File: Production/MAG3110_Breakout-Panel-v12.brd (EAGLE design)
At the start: 123.4 x 123.4 mm, 836 parts, among them U1 MAG31101:1, U10 MAG31101:1, U11 MAG31101:1, U12 MAG31101:1, U13 MAG31101:1, U14 MAG31101:1, U15 MAG31101:1, U16 MAG31101:1, U17 MAG31101:1, U18 MAG31101:1, U19 MAG31101:1, U2 MAG31101:1, U20 MAG31101:1, U21 MAG31101:1, U22 MAG31101:1, U23 MAG31101:1, U24 MAG31101:1, U25 MAG31101:1, U26 MAG31101:1, U27 MAG31101:1, U28 MAG31101:1, U29 MAG31101:1, U3 MAG31101:1, U30 MAG31101:1, U31 MAG31101:1, U32 MAG31101:1, U33 MAG31101:1, U34 MAG31101:1, U35 MAG31101:1, U36 MAG31101:1, U37 MAG31101:1, U38 MAG31101:1, U39 MAG31101:1, U4 MAG31101:1, U40 MAG31101:1, U41 MAG31101:1, U42 MAG31101:1, U43 MAG31101:1, U44 MAG31101:1, U45 MAG31101:1, U46 MAG31101:1, U47 MAG31101:1, U48 MAG31101:1, U49 MAG31101:1, U5 MAG31101:1, U6 MAG31101:1, U7 MAG31101:1, U8 MAG31101:1, U9 MAG31101:1

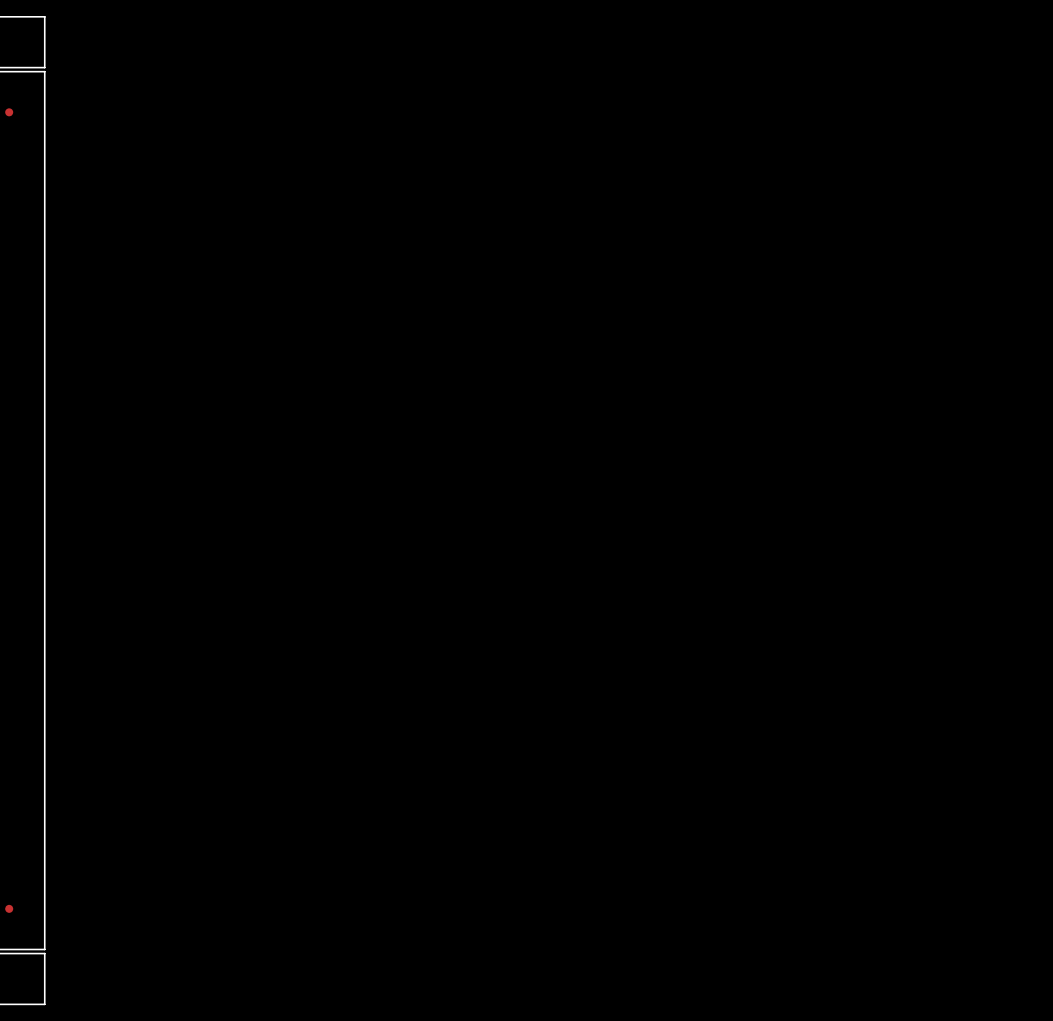
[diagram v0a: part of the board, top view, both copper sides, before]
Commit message: made larger panel
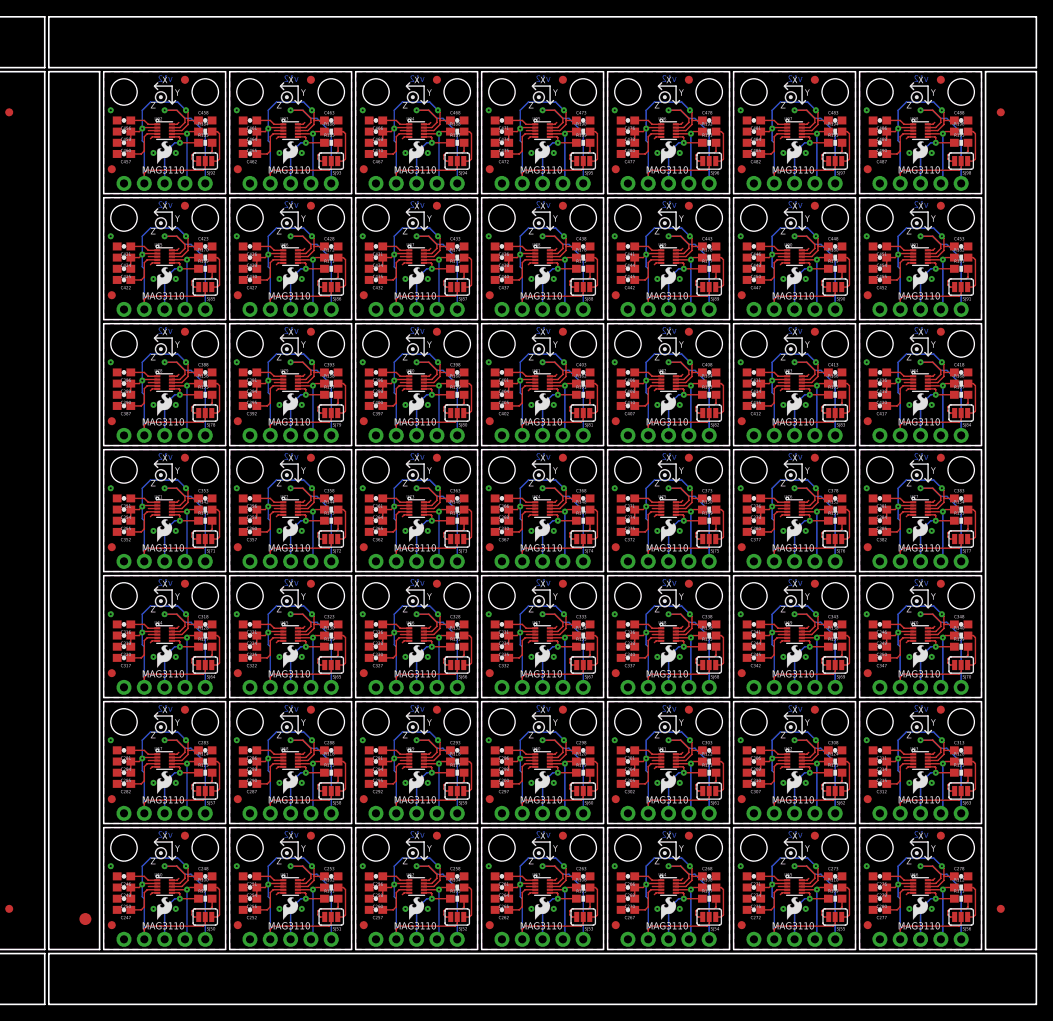
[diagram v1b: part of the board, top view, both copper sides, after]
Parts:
- added C246, C247, C248, C250, C251, C252, C253, C255, C256, C257, C258, C260, C261, C262, C263, C265, C266, C267, C268, C270, C271, C272, C273, C275, C276, C277, C278, C280, C281, C282, C283, C285, C286, C287, C288, C290, C291, C292, C293, C295, C296, C297, C298, C300, C301, C302, C303, C305, C306, C307, C308, C310, C311, C312, C313, C315, C316, C317, C318, C320, C321, C322, C323, C325, C326, C327, C328, C330, C331, C332, C333, C335, C336, C337, C338, C340, C341, C342, C343, C345, C346, C347, C348, C350, C351, C352, C353, C355, C356, C357, C358, C360, C361, C362, C363, C365, C366, C367, C368, C370, C371, C372, C373, C375, C376, C377, C378, C380, C381, C382, C383, C385, C386, C387, C388, C390, C391, C392, C393, C395, C396, C397, C398, C400, C401, C402, C403, C405, C406, C407, C408, C410, C411, C412, C413, C415, C416, C417, C418, C420, C421, C422, C423, C425, C426, C427, C428, C430, C431, C432, C433, C435, C436, C437, C438, C440, C441, C442, C443, C445, C446, C447, C448, C450, C451, C452, C453, C455, C456, C457, C458, C460, C461, C462, C463, C465, C466, C467, C468, C470, C471, C472, C473, C475, C476, C477, C478, C480, C481, C482, C483, C485, C486, C487, C488, C490: 0.1uF, SparkFun:0603-CAP
- added C249, C254, C259, C264, C269, C274, C279, C284, C289, C294, C299, C304, C309, C314, C319, C324, C329, C334, C339, C344, C349, C354, C359, C364, C369, C374, C379, C384, C389, C394, C399, C404, C409, C414, C419, C424, C429, C434, C439, C444, C449, C454, C459, C464, C469, C474, C479, C484, C489: 1uF, SparkFun:0603-CAP
- added E$2, E$3: (no value), SparkFun-Aesthetics:FIDUCIAL-1X2
- added E$5: (no value), SparkFun-Retired:FIDUCIAL-1.5X3
- added FID100, FID101, FID102, FID103, FID104, FID105, FID106, FID107, FID108, FID109, FID110, FID111, FID112, FID113, FID114, FID115, FID116, FID117, FID118, FID119, FID120, FID121, FID122, FID123, FID124, FID125, FID126, FID127, FID128, FID129, FID130, FID131, FID132, FID133, FID134, FID135, FID136, FID137, FID138, FID139, FID140, FID141, FID142, FID143, FID144, FID145, FID146, FID147, FID148, FID149, FID150, FID151, FID152, FID153, FID154, FID155, FID156, FID157, FID158, FID159, FID160, FID161, FID162, FID163, FID164, FID165, FID166, FID167, FID168, FID169, FID170, FID171, FID172, FID173, FID174, FID175, FID176, FID177, FID178, FID179, FID180, FID181, FID182, FID183, FID184, FID185, FID186, FID187, FID188, FID189, FID190, FID191, FID192, FID193, FID194, FID195, FID196, FID99: FIDUCIAL1X2, SparkFun-Aesthetics:FIDUCIAL-1X2
- added JP246, JP251, JP256, JP261, JP266, JP271, JP276, JP281, JP286, JP291, JP296, JP301, JP306, JP311, JP316, JP321, JP326, JP331, JP336, JP341, JP346, JP351, JP356, JP361, JP366, JP371, JP376, JP381, JP386, JP391, JP396, JP401, JP406, JP411, JP416, JP421, JP426, JP431, JP436, JP441, JP446, JP451, JP456, JP461, JP466, JP471, JP476, JP481, JP486: breakout, SparkFun:1X05
- added JP247, JP248, JP252, JP253, JP257, JP258, JP262, JP263, JP267, JP268, JP272, JP273, JP277, JP278, JP282, JP283, JP287, JP288, JP292, JP293, JP297, JP298, JP302, JP303, JP307, JP308, JP312, JP313, JP317, JP318, JP322, JP323, JP327, JP328, JP332, JP333, JP337, JP338, JP342, JP343, JP347, JP348, JP352, JP353, JP357, JP358, JP362, JP363, JP367, JP368, JP372, JP373, JP377, JP378, JP382, JP383, JP387, JP388, JP392, JP393, JP397, JP398, JP402, JP403, JP407, JP408, JP412, JP413, JP417, JP418, JP422, JP423, JP427, JP428, JP432, JP433, JP437, JP438, JP442, JP443, JP447, JP448, JP452, JP453, JP457, JP458, JP462, JP463, JP467, JP468, JP472, JP473, JP477, JP478, JP482, JP483, JP487, JP488: STAND-OFF, SparkFun:STAND-OFF
- added JP249, JP250, JP254, JP255, JP259, JP260, JP264, JP265, JP269, JP270, JP274, JP275, JP279, JP280, JP284, JP285, JP289, JP290, JP294, JP295, JP299, JP300, JP304, JP305, JP309, JP310, JP314, JP315, JP319, JP320, JP324, JP325, JP329, JP330, JP334, JP335, JP339, JP340, JP344, JP345, JP349, JP350, JP354, JP355, JP359, JP360, JP364, JP365, JP369, JP370, JP374, JP375, JP379, JP380, JP384, JP385, JP389, JP390, JP394, JP395, JP399, JP400, JP404, JP405, JP409, JP410, JP414, JP415, JP419, JP420, JP424, JP425, JP429, JP430, JP434, JP435, JP439, JP440, JP444, JP445, JP449, JP450, JP454, JP455, JP459, JP460, JP464, JP465, JP469, JP470, JP474, JP475, JP479, JP480, JP484, JP485, JP489, JP490: LOGO-SFESK, SparkFun:SFE-LOGO-FLAME
- added LOGO50, LOGO51, LOGO52, LOGO53, LOGO54, LOGO55, LOGO56, LOGO57, LOGO58, LOGO59, LOGO60, LOGO61, LOGO62, LOGO63, LOGO64, LOGO65, LOGO66, LOGO67, LOGO68, LOGO69, LOGO70, LOGO71, LOGO72, LOGO73, LOGO74, LOGO75, LOGO76, LOGO77, LOGO78, LOGO79, LOGO80, LOGO81, LOGO82, LOGO83, LOGO84, LOGO85, LOGO86, LOGO87, LOGO88, LOGO89, LOGO90, LOGO91, LOGO92, LOGO93, LOGO94, LOGO95, LOGO96, LOGO97, LOGO98: OSHW-LOGOS, SparkFun-Aesthetics:OSHW-LOGO-S
- added R100, R101, R102, R103, R104, R105, R106, R107, R108, R109, R110, R111, R112, R113, R114, R115, R116, R117, R118, R119, R120, R121, R122, R123, R124, R125, R126, R127, R128, R129, R130, R131, R132, R133, R134, R135, R136, R137, R138, R139, R140, R141, R142, R143, R144, R145, R146, R147, R148, R149, R150, R151, R152, R153, R154, R155, R156, R157, R158, R159, R160, R161, R162, R163, R164, R165, R166, R167, R168, R169, R170, R171, R172, R173, R174, R175, R176, R177, R178, R179, R180, R181, R182, R183, R184, R185, R186, R187, R188, R189, R190, R191, R192, R193, R194, R195, R196, R99: 4.7k, SparkFun:0603-RES
- added SJ50, SJ51, SJ52, SJ53, SJ54, SJ55, SJ56, SJ57, SJ58, SJ59, SJ60, SJ61, SJ62, SJ63, SJ64, SJ65, SJ66, SJ67, SJ68, SJ69, SJ70, SJ71, SJ72, SJ73, SJ74, SJ75, SJ76, SJ77, SJ78, SJ79, SJ80, SJ81, SJ82, SJ83, SJ84, SJ85, SJ86, SJ87, SJ88, SJ89, SJ90, SJ91, SJ92, SJ93, SJ94, SJ95, SJ96, SJ97, SJ98: (no value), SparkFun-Passives:SJ_3_PASTE1&2&3
- added U50, U51, U52, U53, U54, U55, U56, U57, U58, U59, U60, U61, U62, U63, U64, U65, U66, U67, U68, U69, U70, U71, U72, U73, U74, U75, U76, U77, U78, U79, U80, U81, U82, U83, U84, U85, U86, U87, U88, U89, U90, U91, U92, U93, U94, U95, U96, U97, U98: MAG31101:1, SparkFun-Sensors:DFN-10-W
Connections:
- new net GND49: C246.2, C247.2, C248.2, C249.2, C250.2, JP246.1, U50.10, U50.5
- new net GND50: C251.2, C252.2, C253.2, C254.2, C255.2, JP251.1, U51.10, U51.5
- new net GND51: C256.2, C257.2, C258.2, C259.2, C260.2, JP256.1, U52.10, U52.5
- new net GND52: C261.2, C262.2, C263.2, C264.2, C265.2, JP261.1, U53.10, U53.5
- new net GND53: C266.2, C267.2, C268.2, C269.2, C270.2, JP266.1, U54.10, U54.5
- new net GND54: C271.2, C272.2, C273.2, C274.2, C275.2, JP271.1, U55.10, U55.5
- new net GND55: C276.2, C277.2, C278.2, C279.2, C280.2, JP276.1, U56.10, U56.5
- new net GND56: C281.2, C282.2, C283.2, C284.2, C285.2, JP281.1, U57.10, U57.5
- new net GND57: C286.2, C287.2, C288.2, C289.2, C290.2, JP286.1, U58.10, U58.5
- new net GND58: C291.2, C292.2, C293.2, C294.2, C295.2, JP291.1, U59.10, U59.5
- new net GND59: C296.2, C297.2, C298.2, C299.2, C300.2, JP296.1, U60.10, U60.5
- new net GND60: C301.2, C302.2, C303.2, C304.2, C305.2, JP301.1, U61.10, U61.5
- new net GND61: C306.2, C307.2, C308.2, C309.2, C310.2, JP306.1, U62.10, U62.5
- new net GND62: C311.2, C312.2, C313.2, C314.2, C315.2, JP311.1, U63.10, U63.5
- new net GND63: C316.2, C317.2, C318.2, C319.2, C320.2, JP316.1, U64.10, U64.5
- new net GND64: C321.2, C322.2, C323.2, C324.2, C325.2, JP321.1, U65.10, U65.5
- new net GND65: C326.2, C327.2, C328.2, C329.2, C330.2, JP326.1, U66.10, U66.5
- new net GND66: C331.2, C332.2, C333.2, C334.2, C335.2, JP331.1, U67.10, U67.5
- new net GND67: C336.2, C337.2, C338.2, C339.2, C340.2, JP336.1, U68.10, U68.5
- new net GND68: C341.2, C342.2, C343.2, C344.2, C345.2, JP341.1, U69.10, U69.5
- new net GND69: C346.2, C347.2, C348.2, C349.2, C350.2, JP346.1, U70.10, U70.5
- new net GND70: C351.2, C352.2, C353.2, C354.2, C355.2, JP351.1, U71.10, U71.5
- new net GND71: C356.2, C357.2, C358.2, C359.2, C360.2, JP356.1, U72.10, U72.5
- new net GND72: C361.2, C362.2, C363.2, C364.2, C365.2, JP361.1, U73.10, U73.5
- new net GND73: C366.2, C367.2, C368.2, C369.2, C370.2, JP366.1, U74.10, U74.5
- new net GND74: C371.2, C372.2, C373.2, C374.2, C375.2, JP371.1, U75.10, U75.5
- new net GND75: C376.2, C377.2, C378.2, C379.2, C380.2, JP376.1, U76.10, U76.5
- new net GND76: C381.2, C382.2, C383.2, C384.2, C385.2, JP381.1, U77.10, U77.5
- new net GND77: C386.2, C387.2, C388.2, C389.2, C390.2, JP386.1, U78.10, U78.5
- new net GND78: C391.2, C392.2, C393.2, C394.2, C395.2, JP391.1, U79.10, U79.5
- new net GND79: C396.2, C397.2, C398.2, C399.2, C400.2, JP396.1, U80.10, U80.5
- new net GND80: C401.2, C402.2, C403.2, C404.2, C405.2, JP401.1, U81.10, U81.5
- new net GND81: C406.2, C407.2, C408.2, C409.2, C410.2, JP406.1, U82.10, U82.5
- new net GND82: C411.2, C412.2, C413.2, C414.2, C415.2, JP411.1, U83.10, U83.5
- new net GND83: C416.2, C417.2, C418.2, C419.2, C420.2, JP416.1, U84.10, U84.5
- new net GND84: C421.2, C422.2, C423.2, C424.2, C425.2, JP421.1, U85.10, U85.5
- new net GND85: C426.2, C427.2, C428.2, C429.2, C430.2, JP426.1, U86.10, U86.5
- new net GND86: C431.2, C432.2, C433.2, C434.2, C435.2, JP431.1, U87.10, U87.5
- new net GND87: C436.2, C437.2, C438.2, C439.2, C440.2, JP436.1, U88.10, U88.5
- new net GND88: C441.2, C442.2, C443.2, C444.2, C445.2, JP441.1, U89.10, U89.5
- new net GND89: C446.2, C447.2, C448.2, C449.2, C450.2, JP446.1, U90.10, U90.5
- new net GND90: C451.2, C452.2, C453.2, C454.2, C455.2, JP451.1, U91.10, U91.5
- new net GND91: C456.2, C457.2, C458.2, C459.2, C460.2, JP456.1, U92.10, U92.5
- new net GND92: C461.2, C462.2, C463.2, C464.2, C465.2, JP461.1, U93.10, U93.5
- new net GND93: C466.2, C467.2, C468.2, C469.2, C470.2, JP466.1, U94.10, U94.5
- new net GND94: C471.2, C472.2, C473.2, C474.2, C475.2, JP471.1, U95.10, U95.5
- new net GND95: C476.2, C477.2, C478.2, C479.2, C480.2, JP476.1, U96.10, U96.5
- new net GND96: C481.2, C482.2, C483.2, C484.2, C485.2, JP481.1, U97.10, U97.5
- new net GND97: C486.2, C487.2, C488.2, C489.2, C490.2, JP486.1, U98.10, U98.5
- new net INT49: JP246.5, U50.9
- new net INT50: JP251.5, U51.9
- new net INT51: JP256.5, U52.9
- new net INT52: JP261.5, U53.9
- new net INT53: JP266.5, U54.9
- new net INT54: JP271.5, U55.9
- new net INT55: JP276.5, U56.9
- new net INT56: JP281.5, U57.9
- new net INT57: JP286.5, U58.9
- new net INT58: JP291.5, U59.9
- new net INT59: JP296.5, U60.9
- new net INT60: JP301.5, U61.9
- new net INT61: JP306.5, U62.9
- new net INT62: JP311.5, U63.9
- new net INT63: JP316.5, U64.9
- new net INT64: JP321.5, U65.9
- new net INT65: JP326.5, U66.9
- new net INT66: JP331.5, U67.9
- new net INT67: JP336.5, U68.9
- new net INT68: JP341.5, U69.9
- new net INT69: JP346.5, U70.9
- new net INT70: JP351.5, U71.9
- new net INT71: JP356.5, U72.9
- new net INT72: JP361.5, U73.9
- new net INT73: JP366.5, U74.9
- new net INT74: JP371.5, U75.9
- new net INT75: JP376.5, U76.9
- new net INT76: JP381.5, U77.9
- new net INT77: JP386.5, U78.9
- new net INT78: JP391.5, U79.9
- new net INT79: JP396.5, U80.9
- new net INT80: JP401.5, U81.9
- new net INT81: JP406.5, U82.9
- new net INT82: JP411.5, U83.9
- new net INT83: JP416.5, U84.9
- new net INT84: JP421.5, U85.9
- new net INT85: JP426.5, U86.9
- new net INT86: JP431.5, U87.9
- new net INT87: JP436.5, U88.9
- new net INT88: JP441.5, U89.9
- new net INT89: JP446.5, U90.9
- new net INT90: JP451.5, U91.9
- new net INT91: JP456.5, U92.9
- new net INT92: JP461.5, U93.9
- new net INT93: JP466.5, U94.9
- new net INT94: JP471.5, U95.9
- new net INT95: JP476.5, U96.9
- new net INT96: JP481.5, U97.9
- new net INT97: JP486.5, U98.9
- new net N$246: C247.1, U50.4
- new net N$247: C246.1, U50.1
- new net N$248: R100.2, SJ50.1
- new net N$249: R99.2, SJ50.3
- new net N$251: C252.1, U51.4
- new net N$252: C251.1, U51.1
- new net N$253: R102.2, SJ51.1
- new net N$254: R101.2, SJ51.3
- new net N$256: C257.1, U52.4
- new net N$257: C256.1, U52.1
- new net N$258: R104.2, SJ52.1
- new net N$259: R103.2, SJ52.3
- new net N$261: C262.1, U53.4
- new net N$262: C261.1, U53.1
- new net N$263: R106.2, SJ53.1
- new net N$264: R105.2, SJ53.3
- new net N$266: C267.1, U54.4
- new net N$267: C266.1, U54.1
- new net N$268: R108.2, SJ54.1
- new net N$269: R107.2, SJ54.3
- new net N$271: C272.1, U55.4
- new net N$272: C271.1, U55.1
- new net N$273: R110.2, SJ55.1
- new net N$274: R109.2, SJ55.3
- new net N$276: C277.1, U56.4
- new net N$277: C276.1, U56.1
- new net N$278: R112.2, SJ56.1
- new net N$279: R111.2, SJ56.3
- new net N$281: C282.1, U57.4
- new net N$282: C281.1, U57.1
- new net N$283: R114.2, SJ57.1
- new net N$284: R113.2, SJ57.3
- new net N$286: C287.1, U58.4
- new net N$287: C286.1, U58.1
- new net N$288: R116.2, SJ58.1
- new net N$289: R115.2, SJ58.3
- new net N$291: C292.1, U59.4
- new net N$292: C291.1, U59.1
- new net N$293: R118.2, SJ59.1
- new net N$294: R117.2, SJ59.3
- new net N$296: C297.1, U60.4
- new net N$297: C296.1, U60.1
- new net N$298: R120.2, SJ60.1
- new net N$299: R119.2, SJ60.3
- new net N$301: C302.1, U61.4
- new net N$302: C301.1, U61.1
- new net N$303: R122.2, SJ61.1
- new net N$304: R121.2, SJ61.3
- new net N$306: C307.1, U62.4
- new net N$307: C306.1, U62.1
- new net N$308: R124.2, SJ62.1
- new net N$309: R123.2, SJ62.3
- new net N$311: C312.1, U63.4
- new net N$312: C311.1, U63.1
- new net N$313: R126.2, SJ63.1
- new net N$314: R125.2, SJ63.3
- new net N$316: C317.1, U64.4
- new net N$317: C316.1, U64.1
- new net N$318: R128.2, SJ64.1
- new net N$319: R127.2, SJ64.3
- new net N$321: C322.1, U65.4
- new net N$322: C321.1, U65.1
- new net N$323: R130.2, SJ65.1
- new net N$324: R129.2, SJ65.3
- new net N$326: C327.1, U66.4
- new net N$327: C326.1, U66.1
- new net N$328: R132.2, SJ66.1
- new net N$329: R131.2, SJ66.3
- new net N$331: C332.1, U67.4
- new net N$332: C331.1, U67.1
- new net N$333: R134.2, SJ67.1
- new net N$334: R133.2, SJ67.3
- new net N$336: C337.1, U68.4
- new net N$337: C336.1, U68.1
- new net N$338: R136.2, SJ68.1
- new net N$339: R135.2, SJ68.3
- new net N$341: C342.1, U69.4
- new net N$342: C341.1, U69.1
- new net N$343: R138.2, SJ69.1
- new net N$344: R137.2, SJ69.3
- new net N$346: C347.1, U70.4
- new net N$347: C346.1, U70.1
- new net N$348: R140.2, SJ70.1
- new net N$349: R139.2, SJ70.3
- new net N$351: C352.1, U71.4
- new net N$352: C351.1, U71.1
- new net N$353: R142.2, SJ71.1
- new net N$354: R141.2, SJ71.3
- new net N$356: C357.1, U72.4
- new net N$357: C356.1, U72.1
- new net N$358: R144.2, SJ72.1
- new net N$359: R143.2, SJ72.3
- new net N$361: C362.1, U73.4
- new net N$362: C361.1, U73.1
- new net N$363: R146.2, SJ73.1
- new net N$364: R145.2, SJ73.3
- new net N$366: C367.1, U74.4
- new net N$367: C366.1, U74.1
- new net N$368: R148.2, SJ74.1
- new net N$369: R147.2, SJ74.3
- new net N$371: C372.1, U75.4
- new net N$372: C371.1, U75.1
- new net N$373: R150.2, SJ75.1
- new net N$374: R149.2, SJ75.3
- new net N$376: C377.1, U76.4
- new net N$377: C376.1, U76.1
- new net N$378: R152.2, SJ76.1
- new net N$379: R151.2, SJ76.3
- new net N$381: C382.1, U77.4
- new net N$382: C381.1, U77.1
- new net N$383: R154.2, SJ77.1
- new net N$384: R153.2, SJ77.3
- new net N$386: C387.1, U78.4
- new net N$387: C386.1, U78.1
- new net N$388: R156.2, SJ78.1
- new net N$389: R155.2, SJ78.3
- new net N$391: C392.1, U79.4
- new net N$392: C391.1, U79.1
- new net N$393: R158.2, SJ79.1
- new net N$394: R157.2, SJ79.3
- new net N$396: C397.1, U80.4
- new net N$397: C396.1, U80.1
- new net N$398: R160.2, SJ80.1
- new net N$399: R159.2, SJ80.3
- new net N$401: C402.1, U81.4
- new net N$402: C401.1, U81.1
- new net N$403: R162.2, SJ81.1
- new net N$404: R161.2, SJ81.3
- new net N$406: C407.1, U82.4
- new net N$407: C406.1, U82.1
- new net N$408: R164.2, SJ82.1
- new net N$409: R163.2, SJ82.3
- new net N$411: C412.1, U83.4
- new net N$412: C411.1, U83.1
- new net N$413: R166.2, SJ83.1
- new net N$414: R165.2, SJ83.3
- new net N$416: C417.1, U84.4
- new net N$417: C416.1, U84.1
- new net N$418: R168.2, SJ84.1
- new net N$419: R167.2, SJ84.3
- new net N$421: C422.1, U85.4
- new net N$422: C421.1, U85.1
- new net N$423: R170.2, SJ85.1
- new net N$424: R169.2, SJ85.3
- new net N$426: C427.1, U86.4
- new net N$427: C426.1, U86.1
- new net N$428: R172.2, SJ86.1
- new net N$429: R171.2, SJ86.3
- new net N$431: C432.1, U87.4
- new net N$432: C431.1, U87.1
- new net N$433: R174.2, SJ87.1
- new net N$434: R173.2, SJ87.3
- new net N$436: C437.1, U88.4
- new net N$437: C436.1, U88.1
- new net N$438: R176.2, SJ88.1
- new net N$439: R175.2, SJ88.3
- new net N$441: C442.1, U89.4
- new net N$442: C441.1, U89.1
- new net N$443: R178.2, SJ89.1
- new net N$444: R177.2, SJ89.3
- new net N$446: C447.1, U90.4
- new net N$447: C446.1, U90.1
- new net N$448: R180.2, SJ90.1
- new net N$449: R179.2, SJ90.3
- new net N$451: C452.1, U91.4
- new net N$452: C451.1, U91.1
- new net N$453: R182.2, SJ91.1
- new net N$454: R181.2, SJ91.3
- new net N$456: C457.1, U92.4
- new net N$457: C456.1, U92.1
- new net N$458: R184.2, SJ92.1
- new net N$459: R183.2, SJ92.3
- new net N$461: C462.1, U93.4
- new net N$462: C461.1, U93.1
- new net N$463: R186.2, SJ93.1
- new net N$464: R185.2, SJ93.3
- new net N$466: C467.1, U94.4
- new net N$467: C466.1, U94.1
- new net N$468: R188.2, SJ94.1
- new net N$469: R187.2, SJ94.3
- new net N$471: C472.1, U95.4
- new net N$472: C471.1, U95.1
- new net N$473: R190.2, SJ95.1
- new net N$474: R189.2, SJ95.3
- new net N$476: C477.1, U96.4
- new net N$477: C476.1, U96.1
- new net N$478: R192.2, SJ96.1
- new net N$479: R191.2, SJ96.3
- new net N$481: C482.1, U97.4
- new net N$482: C481.1, U97.1
- new net N$483: R194.2, SJ97.1
- new net N$484: R193.2, SJ97.3
- new net N$486: C487.1, U98.4
- new net N$487: C486.1, U98.1
- new net N$488: R196.2, SJ98.1
- new net N$489: R195.2, SJ98.3
- new net SCL49: JP246.4, R100.1, U50.7
- new net SCL50: JP251.4, R102.1, U51.7
- new net SCL51: JP256.4, R104.1, U52.7
- new net SCL52: JP261.4, R106.1, U53.7
- new net SCL53: JP266.4, R108.1, U54.7
- new net SCL54: JP271.4, R110.1, U55.7
- new net SCL55: JP276.4, R112.1, U56.7
- new net SCL56: JP281.4, R114.1, U57.7
- new net SCL57: JP286.4, R116.1, U58.7
- new net SCL58: JP291.4, R118.1, U59.7
- new net SCL59: JP296.4, R120.1, U60.7
- new net SCL60: JP301.4, R122.1, U61.7
- new net SCL61: JP306.4, R124.1, U62.7
- new net SCL62: JP311.4, R126.1, U63.7
- new net SCL63: JP316.4, R128.1, U64.7
- new net SCL64: JP321.4, R130.1, U65.7
- new net SCL65: JP326.4, R132.1, U66.7
- new net SCL66: JP331.4, R134.1, U67.7
- new net SCL67: JP336.4, R136.1, U68.7
- new net SCL68: JP341.4, R138.1, U69.7
- new net SCL69: JP346.4, R140.1, U70.7
- new net SCL70: JP351.4, R142.1, U71.7
- new net SCL71: JP356.4, R144.1, U72.7
- new net SCL72: JP361.4, R146.1, U73.7
- new net SCL73: JP366.4, R148.1, U74.7
- new net SCL74: JP371.4, R150.1, U75.7
- new net SCL75: JP376.4, R152.1, U76.7
- new net SCL76: JP381.4, R154.1, U77.7
- new net SCL77: JP386.4, R156.1, U78.7
- new net SCL78: JP391.4, R158.1, U79.7
- new net SCL79: JP396.4, R160.1, U80.7
- new net SCL80: JP401.4, R162.1, U81.7
- new net SCL81: JP406.4, R164.1, U82.7
- new net SCL82: JP411.4, R166.1, U83.7
- new net SCL83: JP416.4, R168.1, U84.7
- new net SCL84: JP421.4, R170.1, U85.7
- new net SCL85: JP426.4, R172.1, U86.7
- new net SCL86: JP431.4, R174.1, U87.7
- new net SCL87: JP436.4, R176.1, U88.7
- new net SCL88: JP441.4, R178.1, U89.7
- new net SCL89: JP446.4, R180.1, U90.7
- new net SCL90: JP451.4, R182.1, U91.7
- new net SCL91: JP456.4, R184.1, U92.7
- new net SCL92: JP461.4, R186.1, U93.7
- new net SCL93: JP466.4, R188.1, U94.7
- new net SCL94: JP471.4, R190.1, U95.7
- new net SCL95: JP476.4, R192.1, U96.7
- new net SCL96: JP481.4, R194.1, U97.7
- new net SCL97: JP486.4, R196.1, U98.7
- new net SDA49: JP246.3, R99.1, U50.6
- new net SDA50: JP251.3, R101.1, U51.6
- new net SDA51: JP256.3, R103.1, U52.6
- new net SDA52: JP261.3, R105.1, U53.6
- new net SDA53: JP266.3, R107.1, U54.6
- new net SDA54: JP271.3, R109.1, U55.6
- new net SDA55: JP276.3, R111.1, U56.6
- new net SDA56: JP281.3, R113.1, U57.6
- new net SDA57: JP286.3, R115.1, U58.6
- new net SDA58: JP291.3, R117.1, U59.6
- new net SDA59: JP296.3, R119.1, U60.6
- new net SDA60: JP301.3, R121.1, U61.6
- new net SDA61: JP306.3, R123.1, U62.6
- new net SDA62: JP311.3, R125.1, U63.6
- new net SDA63: JP316.3, R127.1, U64.6
- new net SDA64: JP321.3, R129.1, U65.6
- new net SDA65: JP326.3, R131.1, U66.6
- new net SDA66: JP331.3, R133.1, U67.6
- new net SDA67: JP336.3, R135.1, U68.6
- new net SDA68: JP341.3, R137.1, U69.6
- new net SDA69: JP346.3, R139.1, U70.6
- new net SDA70: JP351.3, R141.1, U71.6
- new net SDA71: JP356.3, R143.1, U72.6
- new net SDA72: JP361.3, R145.1, U73.6
- new net SDA73: JP366.3, R147.1, U74.6
- new net SDA74: JP371.3, R149.1, U75.6
- new net SDA75: JP376.3, R151.1, U76.6
- new net SDA76: JP381.3, R153.1, U77.6
- new net SDA77: JP386.3, R155.1, U78.6
- new net SDA78: JP391.3, R157.1, U79.6
- new net SDA79: JP396.3, R159.1, U80.6
- new net SDA80: JP401.3, R161.1, U81.6
- new net SDA81: JP406.3, R163.1, U82.6
- new net SDA82: JP411.3, R165.1, U83.6
- new net SDA83: JP416.3, R167.1, U84.6
- new net SDA84: JP421.3, R169.1, U85.6
- new net SDA85: JP426.3, R171.1, U86.6
- new net SDA86: JP431.3, R173.1, U87.6
- new net SDA87: JP436.3, R175.1, U88.6
- new net SDA88: JP441.3, R177.1, U89.6
- new net SDA89: JP446.3, R179.1, U90.6
- new net SDA90: JP451.3, R181.1, U91.6
- new net SDA91: JP456.3, R183.1, U92.6
- new net SDA92: JP461.3, R185.1, U93.6
- new net SDA93: JP466.3, R187.1, U94.6
- new net SDA94: JP471.3, R189.1, U95.6
- new net SDA95: JP476.3, R191.1, U96.6
- new net SDA96: JP481.3, R193.1, U97.6
- new net SDA97: JP486.3, R195.1, U98.6
- new net VCC49: C248.1, C249.1, C250.1, JP246.2, SJ50.2, U50.2, U50.8
- new net VCC50: C253.1, C254.1, C255.1, JP251.2, SJ51.2, U51.2, U51.8
- new net VCC51: C258.1, C259.1, C260.1, JP256.2, SJ52.2, U52.2, U52.8
- new net VCC52: C263.1, C264.1, C265.1, JP261.2, SJ53.2, U53.2, U53.8
- new net VCC53: C268.1, C269.1, C270.1, JP266.2, SJ54.2, U54.2, U54.8
- new net VCC54: C273.1, C274.1, C275.1, JP271.2, SJ55.2, U55.2, U55.8
- new net VCC55: C278.1, C279.1, C280.1, JP276.2, SJ56.2, U56.2, U56.8
- new net VCC56: C283.1, C284.1, C285.1, JP281.2, SJ57.2, U57.2, U57.8
- new net VCC57: C288.1, C289.1, C290.1, JP286.2, SJ58.2, U58.2, U58.8
- new net VCC58: C293.1, C294.1, C295.1, JP291.2, SJ59.2, U59.2, U59.8
- new net VCC59: C298.1, C299.1, C300.1, JP296.2, SJ60.2, U60.2, U60.8
- new net VCC60: C303.1, C304.1, C305.1, JP301.2, SJ61.2, U61.2, U61.8
- new net VCC61: C308.1, C309.1, C310.1, JP306.2, SJ62.2, U62.2, U62.8
- new net VCC62: C313.1, C314.1, C315.1, JP311.2, SJ63.2, U63.2, U63.8
- new net VCC63: C318.1, C319.1, C320.1, JP316.2, SJ64.2, U64.2, U64.8
- new net VCC64: C323.1, C324.1, C325.1, JP321.2, SJ65.2, U65.2, U65.8
- new net VCC65: C328.1, C329.1, C330.1, JP326.2, SJ66.2, U66.2, U66.8
- new net VCC66: C333.1, C334.1, C335.1, JP331.2, SJ67.2, U67.2, U67.8
- new net VCC67: C338.1, C339.1, C340.1, JP336.2, SJ68.2, U68.2, U68.8
- new net VCC68: C343.1, C344.1, C345.1, JP341.2, SJ69.2, U69.2, U69.8
- new net VCC69: C348.1, C349.1, C350.1, JP346.2, SJ70.2, U70.2, U70.8
- new net VCC70: C353.1, C354.1, C355.1, JP351.2, SJ71.2, U71.2, U71.8
- new net VCC71: C358.1, C359.1, C360.1, JP356.2, SJ72.2, U72.2, U72.8
- new net VCC72: C363.1, C364.1, C365.1, JP361.2, SJ73.2, U73.2, U73.8
- new net VCC73: C368.1, C369.1, C370.1, JP366.2, SJ74.2, U74.2, U74.8
- new net VCC74: C373.1, C374.1, C375.1, JP371.2, SJ75.2, U75.2, U75.8
- new net VCC75: C378.1, C379.1, C380.1, JP376.2, SJ76.2, U76.2, U76.8
- new net VCC76: C383.1, C384.1, C385.1, JP381.2, SJ77.2, U77.2, U77.8
- new net VCC77: C388.1, C389.1, C390.1, JP386.2, SJ78.2, U78.2, U78.8
- new net VCC78: C393.1, C394.1, C395.1, JP391.2, SJ79.2, U79.2, U79.8
- new net VCC79: C398.1, C399.1, C400.1, JP396.2, SJ80.2, U80.2, U80.8
- new net VCC80: C403.1, C404.1, C405.1, JP401.2, SJ81.2, U81.2, U81.8
- new net VCC81: C408.1, C409.1, C410.1, JP406.2, SJ82.2, U82.2, U82.8
- new net VCC82: C413.1, C414.1, C415.1, JP411.2, SJ83.2, U83.2, U83.8
- new net VCC83: C418.1, C419.1, C420.1, JP416.2, SJ84.2, U84.2, U84.8
- new net VCC84: C423.1, C424.1, C425.1, JP421.2, SJ85.2, U85.2, U85.8
- new net VCC85: C428.1, C429.1, C430.1, JP426.2, SJ86.2, U86.2, U86.8
- new net VCC86: C433.1, C434.1, C435.1, JP431.2, SJ87.2, U87.2, U87.8
- new net VCC87: C438.1, C439.1, C440.1, JP436.2, SJ88.2, U88.2, U88.8
- new net VCC88: C443.1, C444.1, C445.1, JP441.2, SJ89.2, U89.2, U89.8
- new net VCC89: C448.1, C449.1, C450.1, JP446.2, SJ90.2, U90.2, U90.8
- new net VCC90: C453.1, C454.1, C455.1, JP451.2, SJ91.2, U91.2, U91.8
- new net VCC91: C458.1, C459.1, C460.1, JP456.2, SJ92.2, U92.2, U92.8
- new net VCC92: C463.1, C464.1, C465.1, JP461.2, SJ93.2, U93.2, U93.8
- new net VCC93: C468.1, C469.1, C470.1, JP466.2, SJ94.2, U94.2, U94.8
- new net VCC94: C473.1, C474.1, C475.1, JP471.2, SJ95.2, U95.2, U95.8
- new net VCC95: C478.1, C479.1, C480.1, JP476.2, SJ96.2, U96.2, U96.8
- new net VCC96: C483.1, C484.1, C485.1, JP481.2, SJ97.2, U97.2, U97.8
- new net VCC97: C488.1, C489.1, C490.1, JP486.2, SJ98.2, U98.2, U98.8
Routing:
- net VCC90: track 0.00 -> 36.0 mm, vias 0 -> 2
- net VCC87: track 0.00 -> 36.0 mm, vias 0 -> 2
- net VCC84: track 0.00 -> 36.0 mm, vias 0 -> 2
- net VCC88: track 0.00 -> 36.0 mm, vias 0 -> 2
- net VCC85: track 0.00 -> 36.0 mm, vias 0 -> 2
- net VCC89: track 0.00 -> 36.0 mm, vias 0 -> 2
- net VCC86: track 0.00 -> 36.0 mm, vias 0 -> 2
- net VCC55: track 0.00 -> 36.0 mm, vias 0 -> 2
- net VCC52: track 0.00 -> 36.0 mm, vias 0 -> 2
- net VCC49: track 0.00 -> 36.0 mm, vias 0 -> 2
- net VCC97: track 0.00 -> 36.0 mm, vias 0 -> 2
- net VCC94: track 0.00 -> 36.0 mm, vias 0 -> 2
- net VCC91: track 0.00 -> 36.0 mm, vias 0 -> 2
- net VCC76: track 0.00 -> 36.0 mm, vias 0 -> 2
- net VCC73: track 0.00 -> 36.0 mm, vias 0 -> 2
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- added copper zone on layer 1, net GND49
- added copper zone on layer 16, net GND49
- added copper zone on layer 1, net GND50
- added copper zone on layer 16, net GND50
- added copper zone on layer 1, net GND51
- added copper zone on layer 16, net GND51
- added copper zone on layer 1, net GND52
- added copper zone on layer 16, net GND52
- added copper zone on layer 1, net GND53
- added copper zone on layer 16, net GND53
- added copper zone on layer 1, net GND54
- added copper zone on layer 16, net GND54
- added copper zone on layer 1, net GND55
- added copper zone on layer 16, net GND55
- added copper zone on layer 1, net GND56
- added copper zone on layer 16, net GND56
- added copper zone on layer 1, net GND57
- added copper zone on layer 16, net GND57
- added copper zone on layer 1, net GND58
- added copper zone on layer 16, net GND58
- added copper zone on layer 1, net GND59
- added copper zone on layer 16, net GND59
- added copper zone on layer 1, net GND60
- added copper zone on layer 16, net GND60
- added copper zone on layer 1, net GND61
- added copper zone on layer 16, net GND61
- added copper zone on layer 1, net GND62
- added copper zone on layer 16, net GND62
- added copper zone on layer 1, net GND63
- added copper zone on layer 16, net GND63
- added copper zone on layer 1, net GND64
- added copper zone on layer 16, net GND64
- added copper zone on layer 1, net GND65
- added copper zone on layer 16, net GND65
- added copper zone on layer 1, net GND66
- added copper zone on layer 16, net GND66
- added copper zone on layer 1, net GND67
- added copper zone on layer 16, net GND67
- added copper zone on layer 1, net GND68
- added copper zone on layer 16, net GND68
- added copper zone on layer 1, net GND69
- added copper zone on layer 16, net GND69
- added copper zone on layer 1, net GND70
- added copper zone on layer 16, net GND70
- added copper zone on layer 1, net GND71
- added copper zone on layer 16, net GND71
- added copper zone on layer 1, net GND72
- added copper zone on layer 16, net GND72
- added copper zone on layer 1, net GND73
- added copper zone on layer 16, net GND73
- added copper zone on layer 1, net GND74
- added copper zone on layer 16, net GND74
- added copper zone on layer 1, net GND75
- added copper zone on layer 16, net GND75
- added copper zone on layer 1, net GND76
- added copper zone on layer 16, net GND76
- added copper zone on layer 1, net GND77
- added copper zone on layer 16, net GND77
- added copper zone on layer 1, net GND78
- added copper zone on layer 16, net GND78
- added copper zone on layer 1, net GND79
- added copper zone on layer 16, net GND79
- added copper zone on layer 1, net GND80
- added copper zone on layer 16, net GND80
- added copper zone on layer 1, net GND81
- added copper zone on layer 16, net GND81
- added copper zone on layer 1, net GND82
- added copper zone on layer 16, net GND82
- added copper zone on layer 1, net GND83
- added copper zone on layer 16, net GND83
- added copper zone on layer 1, net GND84
- added copper zone on layer 16, net GND84
- added copper zone on layer 1, net GND85
- added copper zone on layer 16, net GND85
- added copper zone on layer 1, net GND86
- added copper zone on layer 16, net GND86
- added copper zone on layer 1, net GND87
- added copper zone on layer 16, net GND87
- added copper zone on layer 1, net GND88
- added copper zone on layer 16, net GND88
- added copper zone on layer 1, net GND89
- added copper zone on layer 16, net GND89
- added copper zone on layer 1, net GND90
- added copper zone on layer 16, net GND90
- added copper zone on layer 1, net GND91
- added copper zone on layer 16, net GND91
- added copper zone on layer 1, net GND92
- added copper zone on layer 16, net GND92
- added copper zone on layer 1, net GND93
- added copper zone on layer 16, net GND93
- added copper zone on layer 1, net GND94
- added copper zone on layer 16, net GND94
- added copper zone on layer 1, net GND95
- added copper zone on layer 16, net GND95
- added copper zone on layer 1, net GND96
- added copper zone on layer 16, net GND96
- added copper zone on layer 1, net GND97
- added copper zone on layer 16, net GND97
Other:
- board size 123.4 x 123.4 mm -> 247.4 x 123.4 mm
